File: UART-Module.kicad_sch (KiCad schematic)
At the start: 10 parts, among them J4 DE9_Receptacle_MountingHoles, Q2 1.8432, U1 74HC02, U2 74HC21, U3 W65C21N, U5 R65C51

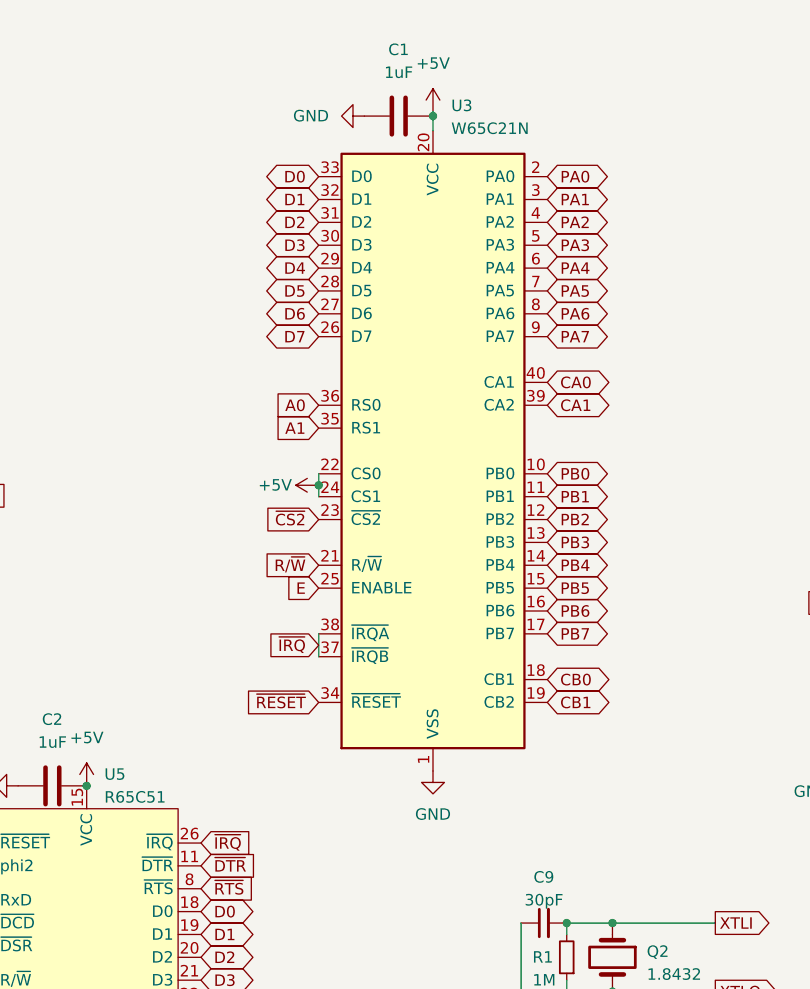
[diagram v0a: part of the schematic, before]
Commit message: revise components
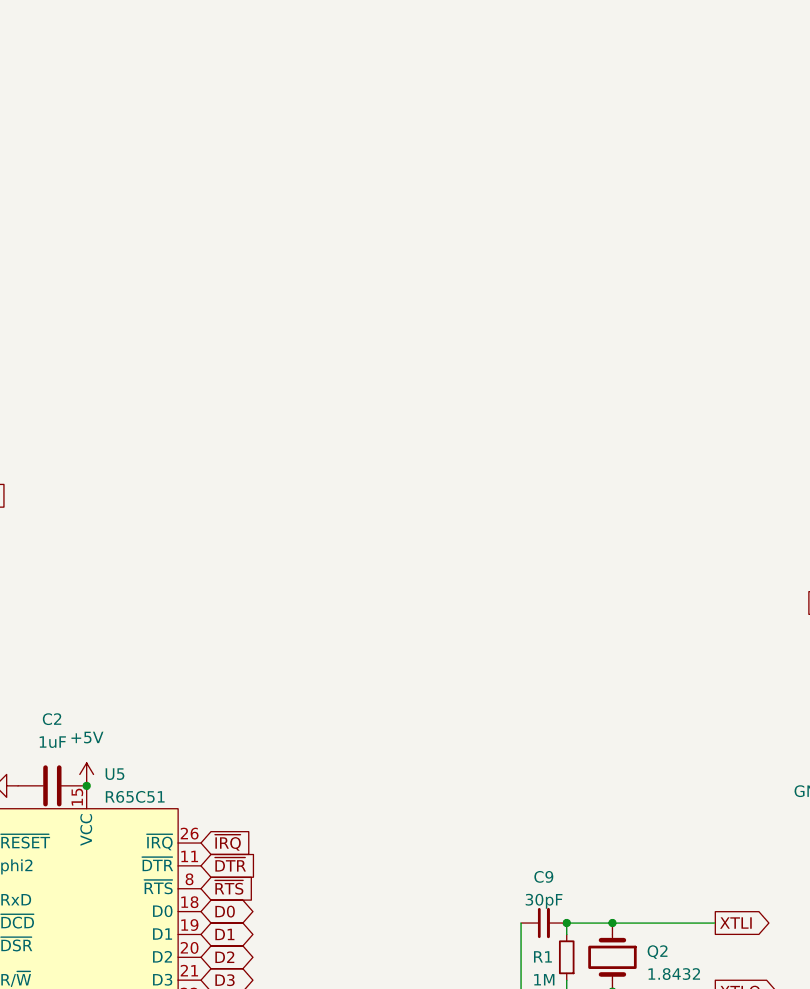
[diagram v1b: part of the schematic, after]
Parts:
- removed C1: 1uF, Capacitor_SMD:C_0805_2012Metric, symbol Device:C
- removed U3: W65C21N, Package_DIP:DIP-40_W15.24mm, symbol Interface:6821
